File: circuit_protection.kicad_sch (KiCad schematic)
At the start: 39 parts, among them IC2 TPS26632RGET, Q5 2N7002, Q6 CSD19537Q3, U10 USBLC6-2SC6, U11 USBLC6-2SC6, U13 MAX40200AUK, U2 SEUC10F5V4U, U3 TPS259630DDAR, U8 USBLC6-2SC6

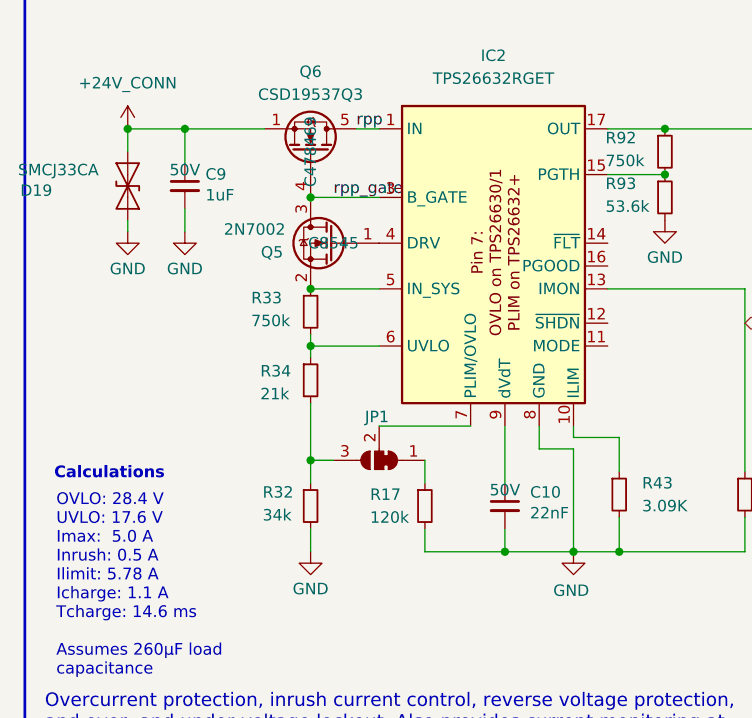
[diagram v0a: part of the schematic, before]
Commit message: MOAR STITCHING and some cleanup
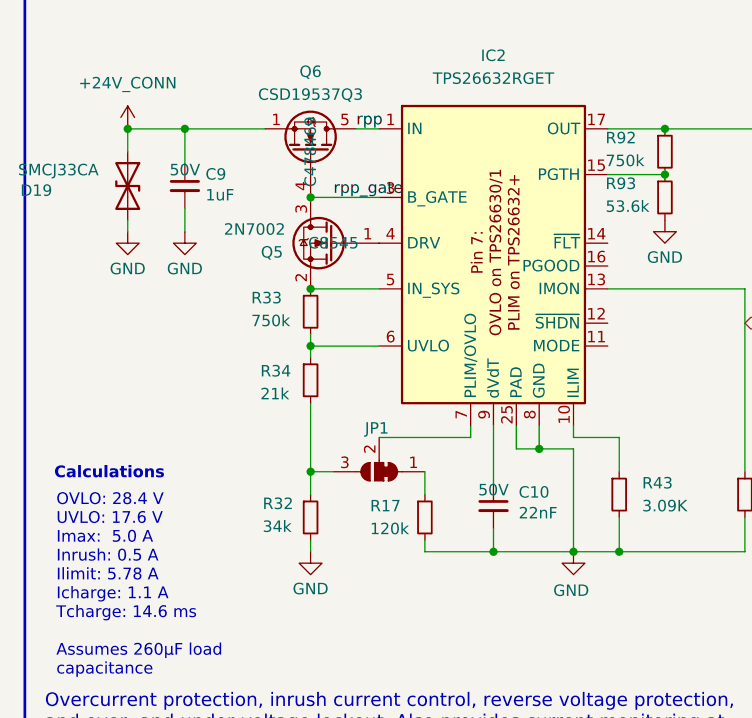
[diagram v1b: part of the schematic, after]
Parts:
- D19: footprint Diode_SMD:D_SMA -> Diode_SMD:D_SMC; symbol Diode:SMAJ5.0CA -> Device:D_TVS
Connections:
- net GND: now also IC2.25 (PAD)
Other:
- moved on the sheet: C10, JP1, R17, R32
